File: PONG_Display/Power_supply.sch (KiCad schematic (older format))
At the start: 0 parts

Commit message: V2
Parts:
- added C?: 470u, symbol Device:CP
- added C?: 100n, symbol Device:C
- added C?: 10u, symbol Device:C
- added C?: 100n, symbol Device:CP
- added J?: Input_Supply+12V, symbol Connector_Generic:Conn_01x02
- added U?: LD1117S33TR_SOT223, Package_TO_SOT_SMD:SOT-223-3_TabPin2, symbol Regulator_Linear:LD1117S33TR_SOT223
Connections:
- new net +12V: J?.1 (Pin_1)
- new net +3V3: C?.1, C?.1, U?.2 (VO)
- new net +5V: C?.1, C?.1, U?.3 (VI)
- new net GND: C?.2, C?.2, C?.2, C?.2, J?.2 (Pin_2), U?.1 (GND)
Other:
- note added: "Schemat układu zasilania"
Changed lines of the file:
@@
 $Descr A4 11693 8268
 encoding utf-8
-Sheet 3 7
+Sheet 6 6
 Title ""
 Date ""
@@
 Comment4 ""
 $EndDescr
+$Comp
+L Connector_Generic:Conn_01x02 J?
+U 1 1 5E83DA30
+P 1750 1750
+AR Path="/5E80CCDD/5E83DA30" Ref="J?"  Part="1"
+AR Path="/5E80B14C/5E83DA30" Ref="J?"  Part="1"
+AR Path="/5E83DA30" Ref="J?"  Part="1"
+F 0 "J?" H 1668 1967 50  0000 C CNN
+F 1 "Input_Supply+12V" H 1668 1876 50  0000 C CNN
+F 2 "" H 1750 1750 50  0001 C CNN
+F 3 "~" H 1750 1750 50  0001 C CNN
+	1    1750 1750
+	-1   0    0    -1
+$EndComp
+Text Notes 7850 7500 0    50   ~ 0
+Schemat układu zasilania
+$Comp
+L power:+12V #PWR?
+U 1 1 5E85C905
+P 2400 1600
+F 0 "#PWR?" H 2400 1450 50  0001 C CNN
+F 1 "+12V" H 2415 1773 50  0000 C CNN
+F 2 "" H 2400 1600 50  0001 C CNN
+F 3 "" H 2400 1600 50  0001 C CNN
+	1    2400 1600
+	-1   0    0    -1
+$EndComp
+$Comp
+L power:GND #PWR?
+U 1 1 5E85CD82
+P 2400 2000
+F 0 "#PWR?" H 2400 1750 50  0001 C CNN
+F 1 "GND" H 2405 1827 50  0000 C CNN
+F 2 "" H 2400 2000 50  0001 C CNN
+F 3 "" H 2400 2000 50  0001 C CNN
+	1    2400 2000
+	-1   0    0    -1
+$EndComp
+Wire Wire Line
+	2400 1600 2400 1750
+Wire Wire Line
+	2400 1750 1950 1750
+Wire Wire Line
+	2400 1850 2400 2000
+Wire Wire Line
+	2400 1850 1950 1850
+$Comp
+L Regulator_Linear:LD1117S33TR_SOT223 U?
+U 1 1 5E860E17
+P 8200 1650
+F 0 "U?" H 8200 1892 50  0000 C CNN
+F 1 "LD1117S33TR_SOT223" H 8200 1801 50  0000 C CNN
+F 2 "Package_TO_SOT_SMD:SOT-223-3_TabPin2" H 8200 1850 50  0001 C CNN
+F 3 "http://www.st.com/st-web-ui/static/active/en/resource/technical/document/datasheet/CD00000544.pdf" H 8300 1400 50  0001 C CNN
+	1    8200 1650
+	1    0    0    -1
+$EndComp
+$Comp
+L power:GND #PWR?
+U 1 1 5E862C71
+P 8200 2100
+F 0 "#PWR?" H 8200 1850 50  0001 C CNN
+F 1 "GND" H 8205 1927 50  0000 C CNN
+F 2 "" H 8200 2100 50  0001 C CNN
+F 3 "" H 8200 2100 50  0001 C CNN
+	1    8200 2100
+	1    0    0    -1
+$EndComp
+$Comp
+L power:+5V #PWR?
+U 1 1 5E862F46
+P 7000 1500
+F 0 "#PWR?" H 7000 1350 50  0001 C CNN
+F 1 "+5V" H 7015 1673 50  0000 C CNN
+F 2 "" H 7000 1500 50  0001 C CNN
+F 3 "" H 7000 1500 50  0001 C CNN
+	1    7000 1500
+	1    0    0    -1
+$EndComp
+$Comp
+L power:+3.3V #PWR?
+U 1 1 5E8636C0
+P 9300 1500
+F 0 "#PWR?" H 9300 1350 50  0001 C CNN
+F 1 "+3.3V" H 9315 1673 50  0000 C CNN
+F 2 "" H 9300 1500 50  0001 C CNN
+F 3 "" H 9300 1500 50  0001 C CNN
+	1    9300 1500
+	1    0    0    -1
+$EndComp
+Wire Wire Line
+	8200 1950 8200 2100
+Wire Wire Line
+	8500 1650 8700 1650
+Wire Wire Line
+	9300 1650 9300 1500
+Wire Wire Line
+	7000 1500 7000 1650
+Wire Wire Line
+	7000 1650 7200 1650
+$Comp
+L Device:CP C?
+U 1 1 5E864BF2
+P 7200 1900
+F 0 "C?" H 7318 1946 50  0000 L CNN
+F 1 "470u" H 7318 1855 50  0000 L CNN
+F 2 "" H 7238 1750 50  0001 C CNN
+F 3 "~" H 7200 1900 50  0001 C CNN
+	1    7200 1900
+	1    0    0    -1
+$EndComp
+$Comp
+L Device:C C?
+U 1 1 5E86541E
+P 7600 1900
+F 0 "C?" H 7715 1946 50  0000 L CNN
+F 1 "100n" H 7715 1855 50  0000 L CNN
+F 2 "" H 7638 1750 50  0001 C CNN
+F 3 "~" H 7600 1900 50  0001 C CNN
+	1    7600 1900
+	1    0    0    -1
+$EndComp
+$Comp
+L Device:C C?
+U 1 1 5E8658D9
+P 8700 1900
+F 0 "C?" H 8815 1946 50  0000 L CNN
+F 1 "10u" H 8815 1855 50  0000 L CNN
+F 2 "" H 8738 1750 50  0001 C CNN
+F 3 "~" H 8700 1900 50  0001 C CNN
+	1    8700 1900
+	1    0    0    -1
+$EndComp
+$Comp
+L Device:CP C?
+U 1 1 5E8660CC
+P 9050 1900
+F 0 "C?" H 9168 1946 50  0000 L CNN
+F 1 "100n" H 9168 1855 50  0000 L CNN
+F 2 "" H 9088 1750 50  0001 C CNN
+F 3 "~" H 9050 1900 50  0001 C CNN
+	1    9050 1900
+	1    0    0    -1
+$EndComp
+$Comp
+L power:GND #PWR?
+U 1 1 5E866491
+P 7200 2150
+F 0 "#PWR?" H 7200 1900 50  0001 C CNN
+F 1 "GND" H 7205 1977 50  0000 C CNN
+F 2 "" H 7200 2150 50  0001 C CNN
+F 3 "" H 7200 2150 50  0001 C CNN
+	1    7200 2150
+	1    0    0    -1
+$EndComp
+$Comp
+L power:GND #PWR?
+U 1 1 5E8668A3
+P 7600 2150
+F 0 "#PWR?" H 7600 1900 50  0001 C CNN
+F 1 "GND" H 7605 1977 50  0000 C CNN
+F 2 "" H 7600 2150 50  0001 C CNN
+F 3 "" H 7600 2150 50  0001 C CNN
+	1    7600 2150
+	1    0    0    -1
+$EndComp
+$Comp
+L power:GND #PWR?
+U 1 1 5E866DAE
+P 8700 2150
+F 0 "#PWR?" H 8700 1900 50  0001 C CNN
+F 1 "GND" H 8705 1977 50  0000 C CNN
+F 2 "" H 8700 2150 50  0001 C CNN
+F 3 "" H 8700 2150 50  0001 C CNN
+	1    8700 2150
+	1    0    0    -1
+$EndComp
+$Comp
+L power:GND #PWR?
+U 1 1 5E8670D0
+P 9050 2150
+F 0 "#PWR?" H 9050 1900 50  0001 C CNN
+F 1 "GND" H 9055 1977 50  0000 C CNN
+F 2 "" H 9050 2150 50  0001 C CNN
+F 3 "" H 9050 2150 50  0001 C CNN
+	1    9050 2150
+	1    0    0    -1
+$EndComp
+Wire Wire Line
+	9050 2050 9050 2150
+Wire Wire Line
+	8700 2050 8700 2150
+Wire Wire Line
+	7600 2050 7600 2150
+Wire Wire Line
+	7200 2050 7200 2150
+Wire Wire Line
+	7200 1650 7200 1750
+Connection ~ 7200 1650
+Wire Wire Line
+	7200 1650 7600 1650
+Wire Wire Line
+	7600 1650 7600 1750
+Connection ~ 7600 1650
+Wire Wire Line
+	7600 1650 7900 1650
+Wire Wire Line
+	8700 1650 8700 1750
+Connection ~ 8700 1650
+Wire Wire Line
+	8700 1650 9050 1650
+Wire Wire Line
+	9050 1650 9050 1750
+Connection ~ 9050 1650
+Wire Wire Line
+	9050 1650 9300 1650
 $EndSCHEMATC

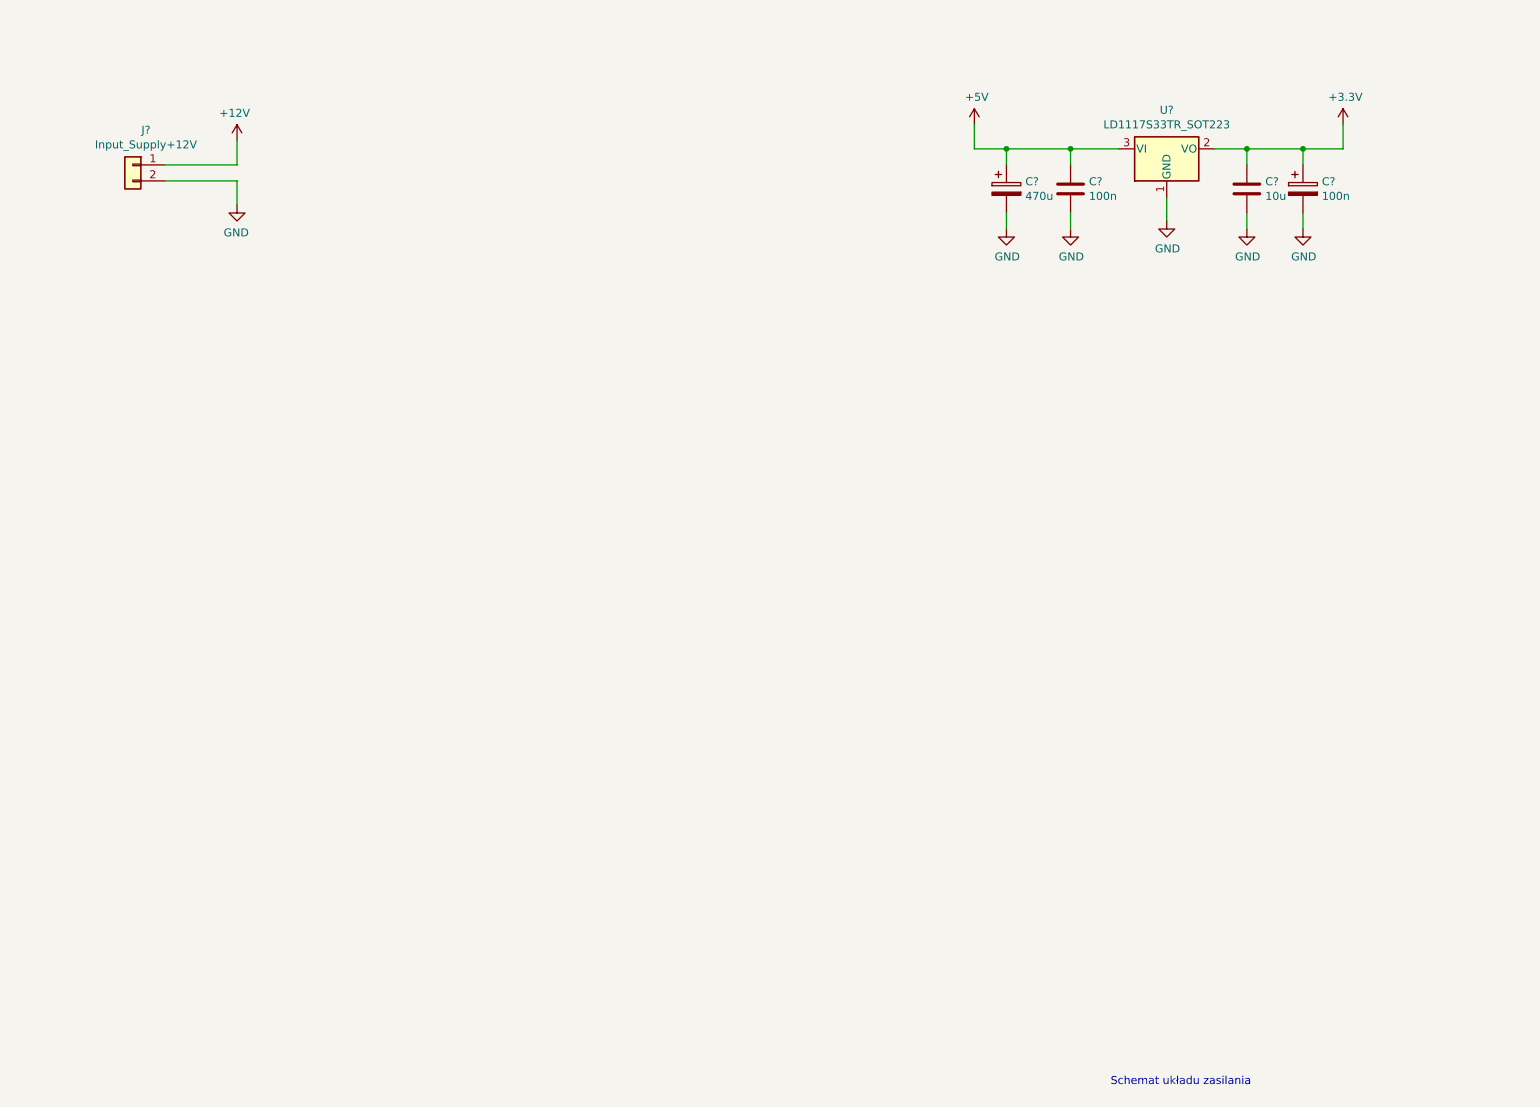
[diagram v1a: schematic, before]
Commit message: V3
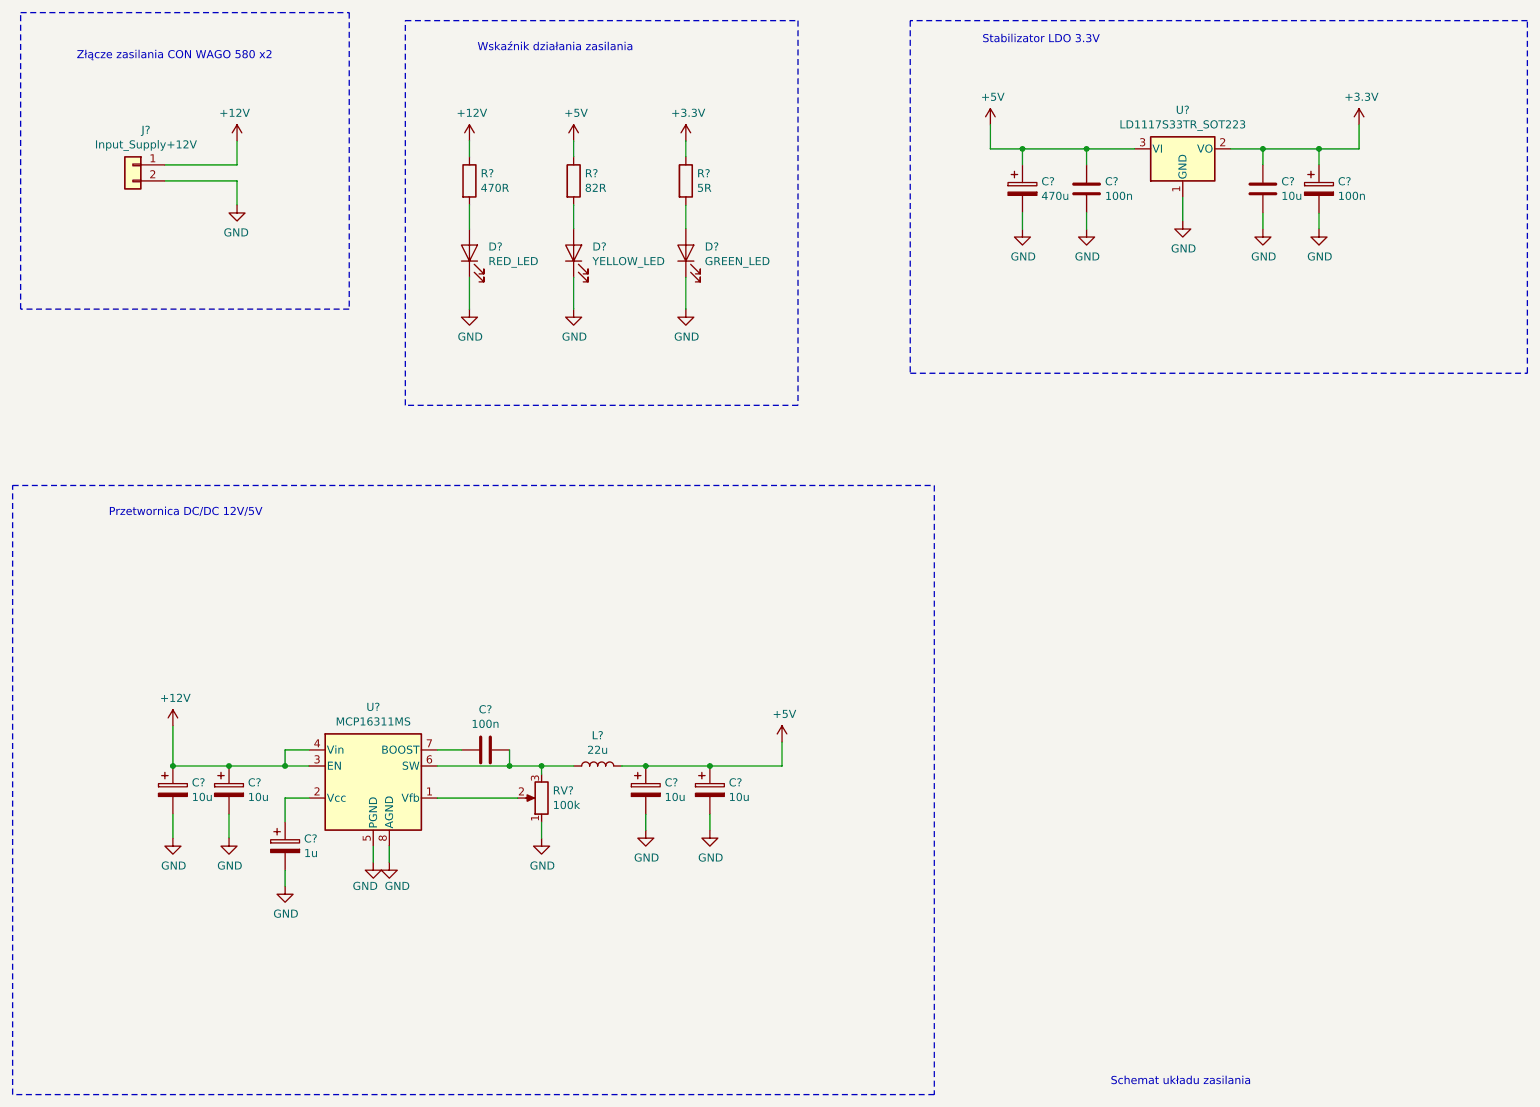
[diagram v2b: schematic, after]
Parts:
- added C?: 1u, symbol Device:CP
- added C? (x4): 10u, symbol Device:CP
- added C?: 100n, symbol Device:C
- added D?: RED_LED, symbol Device:LED
- added D?: YELLOW_LED, symbol Device:LED
- added D?: GREEN_LED, symbol Device:LED
- added L?: 22u, symbol Device:L
- added R?: 470R, symbol Device:R
- added R?: 82R, symbol Device:R
- added R?: 5R, symbol Device:R
- added RV?: 100k, symbol Device:R_POT
- added U?: MCP16311MS, Package_SO:MSOP-8_3x3mm_P0.65mm, symbol Regulator_Switching:MCP16311MS
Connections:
- net +12V: now also C?.1, C?.1, R?.1, U?.3 (EN), U?.4 (Vin)
- net +3V3: now also R?.1
- net +5V: now also C?.1, C?.1, L?.2, R?.1
- net GND: now also C?.2, C?.2, C?.2, C?.2, C?.2, D?.1 (K), D?.1 (K), D?.1 (K), RV?.1, U?.5 (PGND), U?.8 (AGND)
- new net: D?.2 (A), R?.2 (x3)
- new net: RV?.2, U?.1 (Vfb)
- new net: C?.1, U?.2 (Vcc)
- new net: C?.2, L?.1, RV?.3, U?.6 (SW)
- new net: C?.1, U?.7 (BOOST)
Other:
- note added: "Przetwornica DC/DC 12V/5V"
- note added: "Stabilizator LDO 3.3V"
- note added: "Wskaźnik działania zasilania"
- note added: "Złącze zasilania CON WAGO 580 x2"
- moved on the sheet: C?, U?
